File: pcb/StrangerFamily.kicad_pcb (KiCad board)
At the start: 2 copper layers, 90 x 50 mm, 26 parts, among them J1 LCD_Conn, J2 Power_LEDs, J3 Output_LED, J4 LED_Out2, J5 Raspberry_Pi_zero, J6 LED_Out2, Q2 BSS138, Q3 BSS138, Q4 BSS138, U1 74LVC2T45DC, U2 74LVC1G3157

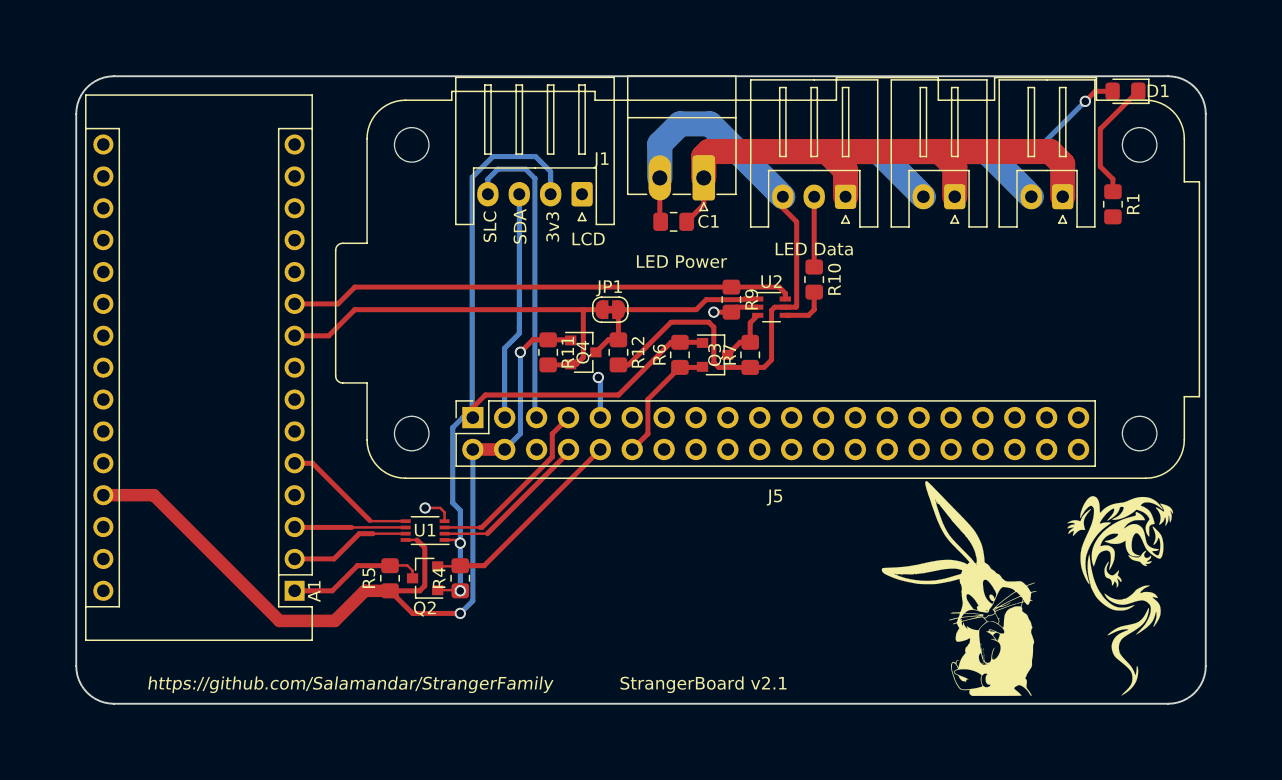
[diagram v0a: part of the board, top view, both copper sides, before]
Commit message: Update kicad project version
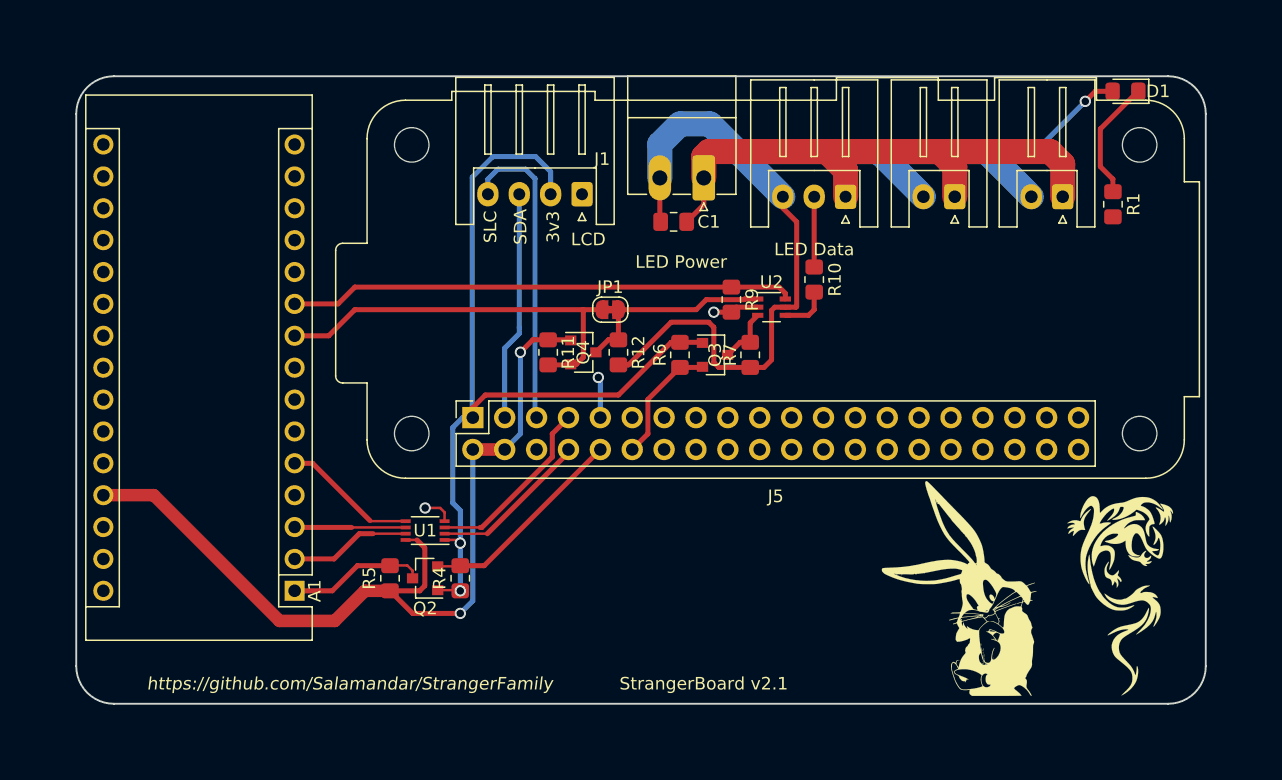
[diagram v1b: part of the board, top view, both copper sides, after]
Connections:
- net /Nano_~Reset renamed /Nano_~{Reset}
- net /RPi_Nano_~Reset renamed /RPi_Nano_~{Reset}
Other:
- net class Default removed
- net class Power removed
